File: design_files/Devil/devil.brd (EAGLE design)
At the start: 24.9 x 23.5 mm, 6 parts

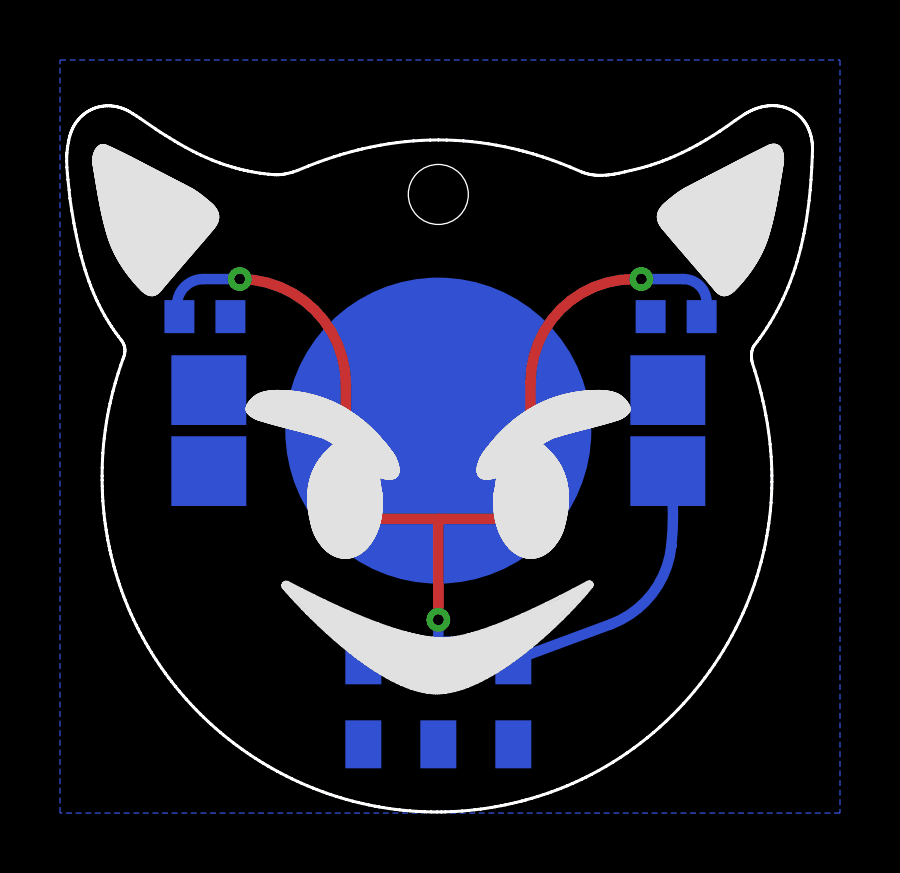
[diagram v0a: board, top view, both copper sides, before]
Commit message: adds updates and pics
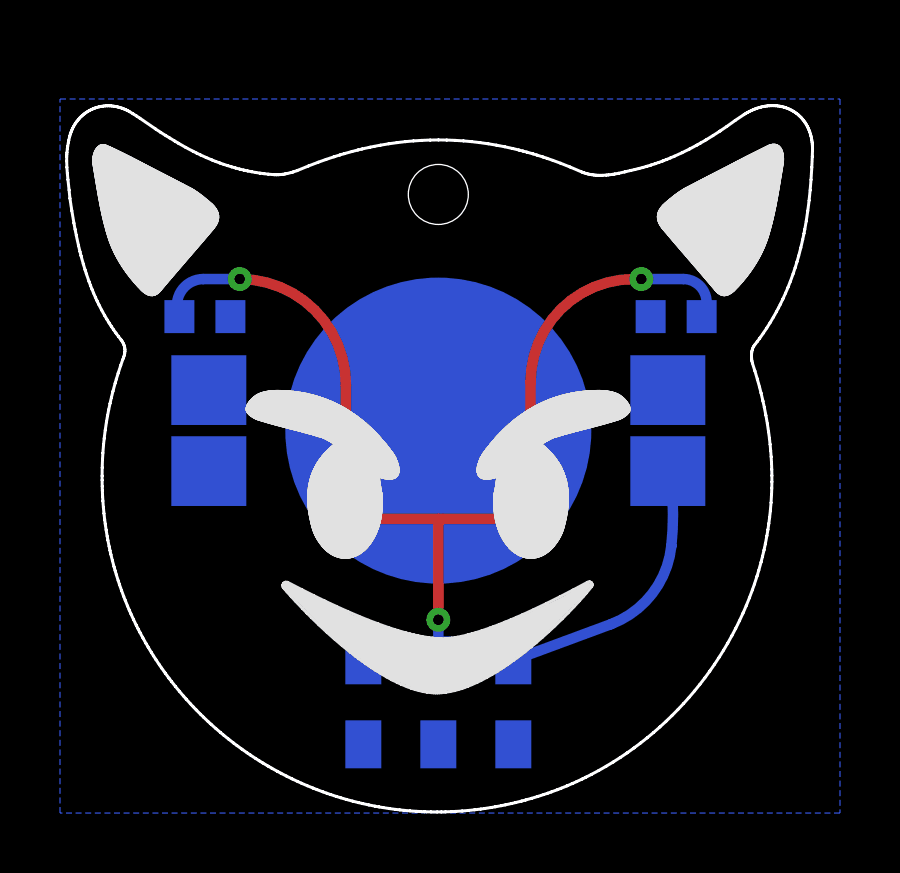
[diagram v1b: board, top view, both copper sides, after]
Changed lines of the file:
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@@
 <drawing>
 <settings>
-<setting alwaysvectorfont="yes"/>
+<setting alwaysvectorfont="no"/>
 <setting verticaltext="up"/>
 </settings>
@@
 </layers>
 <board>
-<fusionsync huburn="a.cGVyc29uYWw6dWUyZGJiODU3" projecturn="a.cGVyc29uYWw6dWUyZGJiODU3IzIwMTkwMTE2MTcwNjgyOTI2" f3durn="urn:adsk.wipprod:dm.lineage:OdxcjZ_0S0ezXZBnbosQ5Q" pcbguid="11cdee58-e33f-4866-a309-80e6dbda0822" lastpulledtime="" lastsyncedchangeguid="4214f7c0-6f33-dc19-8cf7-ab24378442ec"/>
+<fusionsync huburn="a.cGVyc29uYWw6dWUyYzY4MzUz" projecturn="a.cGVyc29uYWw6dWUyYzY4MzUzI0QyMDE5MDQwMzE4NjEyNjk4MQ" f3durn="urn:adsk.wipprod:dm.lineage:VPmSnAdLQfGqMDIWLTXgpg" pcbguid="d5d3fe3d-d1bc-43b6-b4b8-5aa695b34219" lastpulledtime="" lastsyncedchangeguid="94bf7ccc-8d0d-05bc-43fa-d465ada9e75e"/>
 <plain>
 <wire x1="1.225315625" y1="11.23725" x2="1.22874375" y2="11.51538125" width="0.1" layer="20"/>
@@
 <wire x1="23.5137125" y1="22.246846875" x2="23.4483125" y2="22.22378125" width="0.1" layer="49"/>
 <hole x="12.4328" y="20.62" drill="2"/>
+<dimension x1="-0.1778" y1="0" x2="-0.1778" y2="23.8016" x3="-1.1" y3="11.9008" textsize="1.778" layer="1"/>
+<dimension x1="25.8222" y1="0" x2="-0.1778" y2="0" x3="12.8222" y3="-0.1" textsize="1.778" layer="1"/>
 </plain>
 <attributes>
@@
 <attribute name="VALUE" x="20.9956" y="14.6423" size="1.27" layer="28" rot="MR0"/>
 </element>
-<element name="VBAT" library="SamacSys_Parts" package="BATHLD012SMT" override_package3d_urn="urn:adsk.eagle:package:15679619/3" override_package_urn="urn:adsk.eagle:footprint:15679620/1" override_locally_modified="yes" value="BAT-HLD-012-SMT" x="12.4328" y="12.7478" smashed="yes" rot="MR0">
+<element name="VBAT" library="SamacSys_Parts" package="BATHLD012SMT" override_package3d_urn="urn:adsk.eagle:package:32568294/2" override_package_urn="urn:adsk.eagle:footprint:32568295/1" value="BAT-HLD-012-SMT" x="12.4328" y="12.7478" smashed="yes" rot="MR0">
 <attribute name="DESCRIPTION" value="Coin Cell Battery Holders Bat Hld CR1216/1225 Surface Mount" x="12.4328" y="12.7478" size="1.778" layer="28" rot="MR0" display="off"/>
 <attribute name="HEIGHT" value="3mm" x="12.4328" y="12.7478" size="1.778" layer="28" rot="MR0" display="off"/>
@@
 <attribute name="MOUSER_PRICE-STOCK" value="https://www.mouser.com/Search/Refine.aspx?Keyword=712-BAT-HLD-012-SMT" x="12.4328" y="12.7478" size="1.778" layer="28" rot="MR0" display="off"/>
 </element>
-<element name="U$1" library="electroninks" package="CL-SB-22A-02T-DPDT-COMPACT-SWITCH" value="CL-SB-22A-02T-SLIDE-SWITCH-TUCKED-PADS" x="12.4328" y="3.691" smashed="yes" rot="MR0"/>
+<element name="U$1" library="electroninks" package="CL-SB-22A-02T-DPDT-COMPACT-SWITCH" override_package3d_urn="urn:adsk.eagle:package:32569019/2" override_package_urn="urn:adsk.eagle:footprint:32569020/1" value="CL-SB-22A-02T-SLIDE-SWITCH-TUCKED-PADS" x="12.4328" y="3.691" smashed="yes" rot="MR0"/>
 </elements>
 <signals>
@@
 <contactref element="VBAT" pad="P$1"/>
 <polygon width="0.5" layer="16">
-<vertex x="-0.1778" y="25.1016"/>
-<vertex x="25.8222" y="25.1016"/>
+<vertex x="-0.1778" y="23.8016"/>
+<vertex x="25.8222" y="23.8016"/>
 <vertex x="25.8222" y="0"/>
 <vertex x="-0.1778" y="0"/>
 </polygon>
-<wire x1="12.4328" y1="12.7478" x2="19.5106" y2="16.5473" width="0" layer="19" extent="16-16"/>
-<wire x1="5.5026" y1="16.5473" x2="12.4328" y2="12.7478" width="0" layer="19" extent="16-16"/>
 </signal>
 <signal name="VCC">
